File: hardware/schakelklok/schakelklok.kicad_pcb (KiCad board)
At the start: 2 copper layers, 35 parts, among them J1 UART_interface, J2 schakeluitgangen, J3 programmer_1, J4 programmer_2, Q1 BD439, Q2 BD439, Q3 BD439, Q4 BD439, Q5 BD439, SW1 Rotary_Encoder_Switch, U1 24LC64, U2 stm32_bluepill, U3 nrf24l01

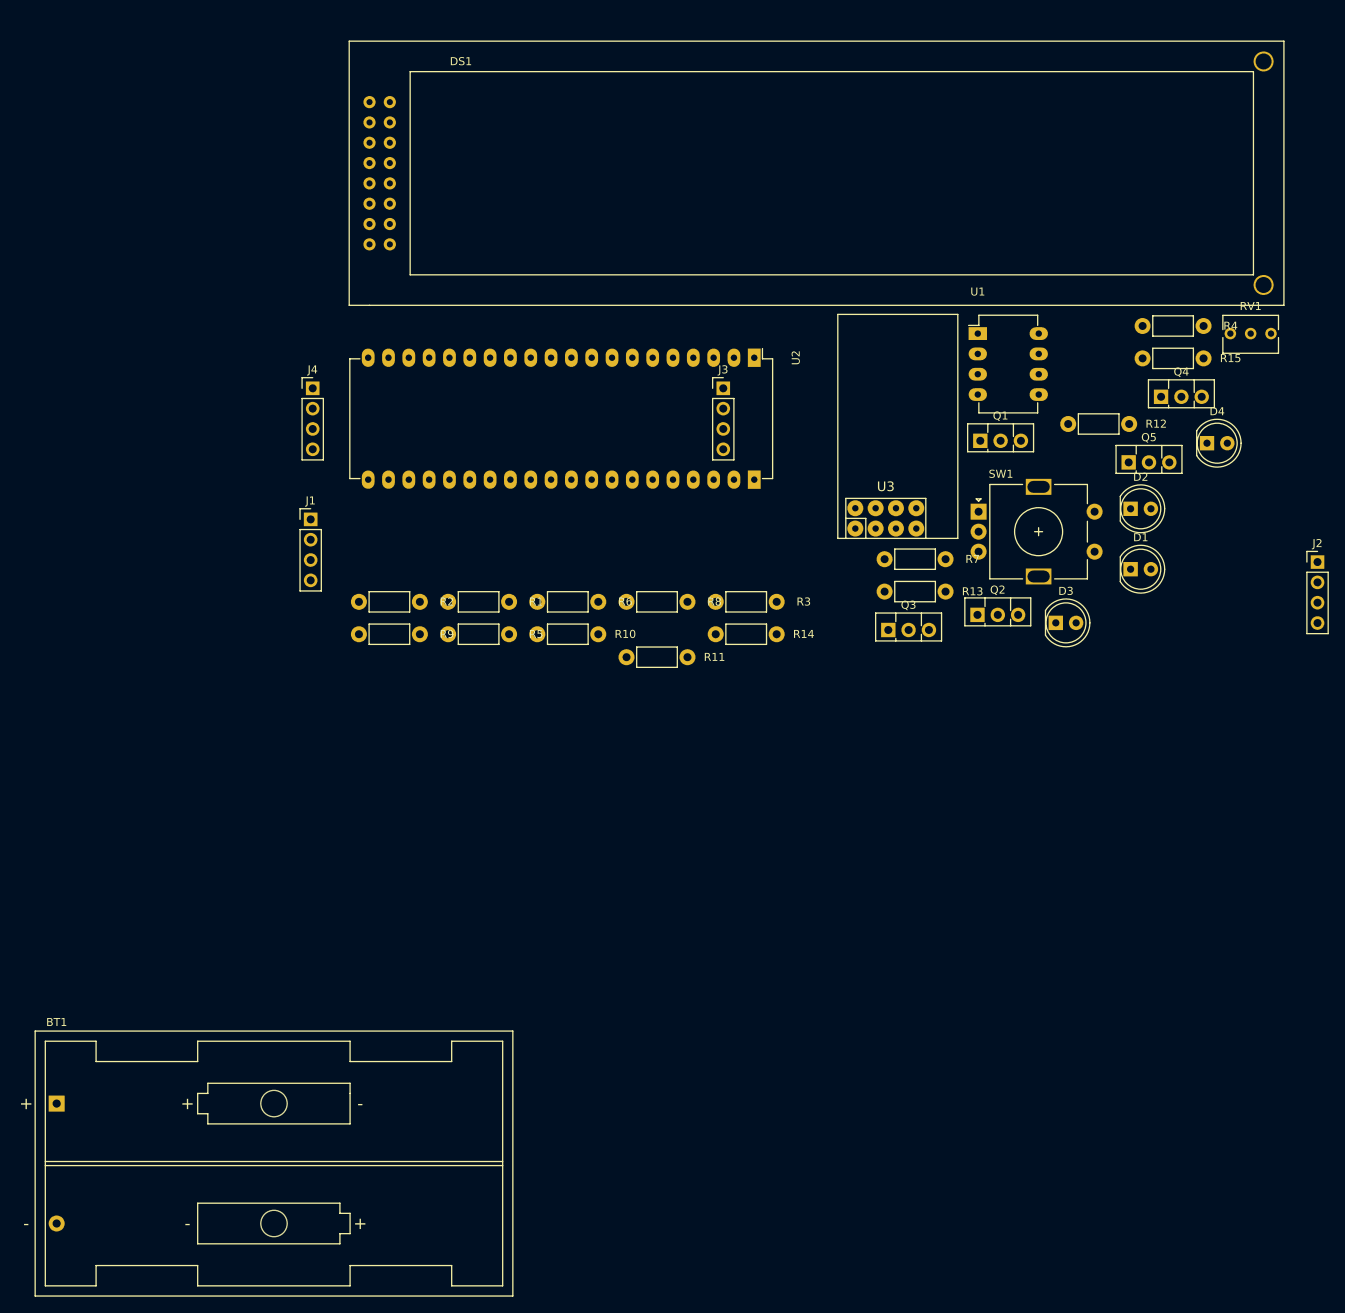
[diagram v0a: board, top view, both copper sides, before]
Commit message: finished hardware
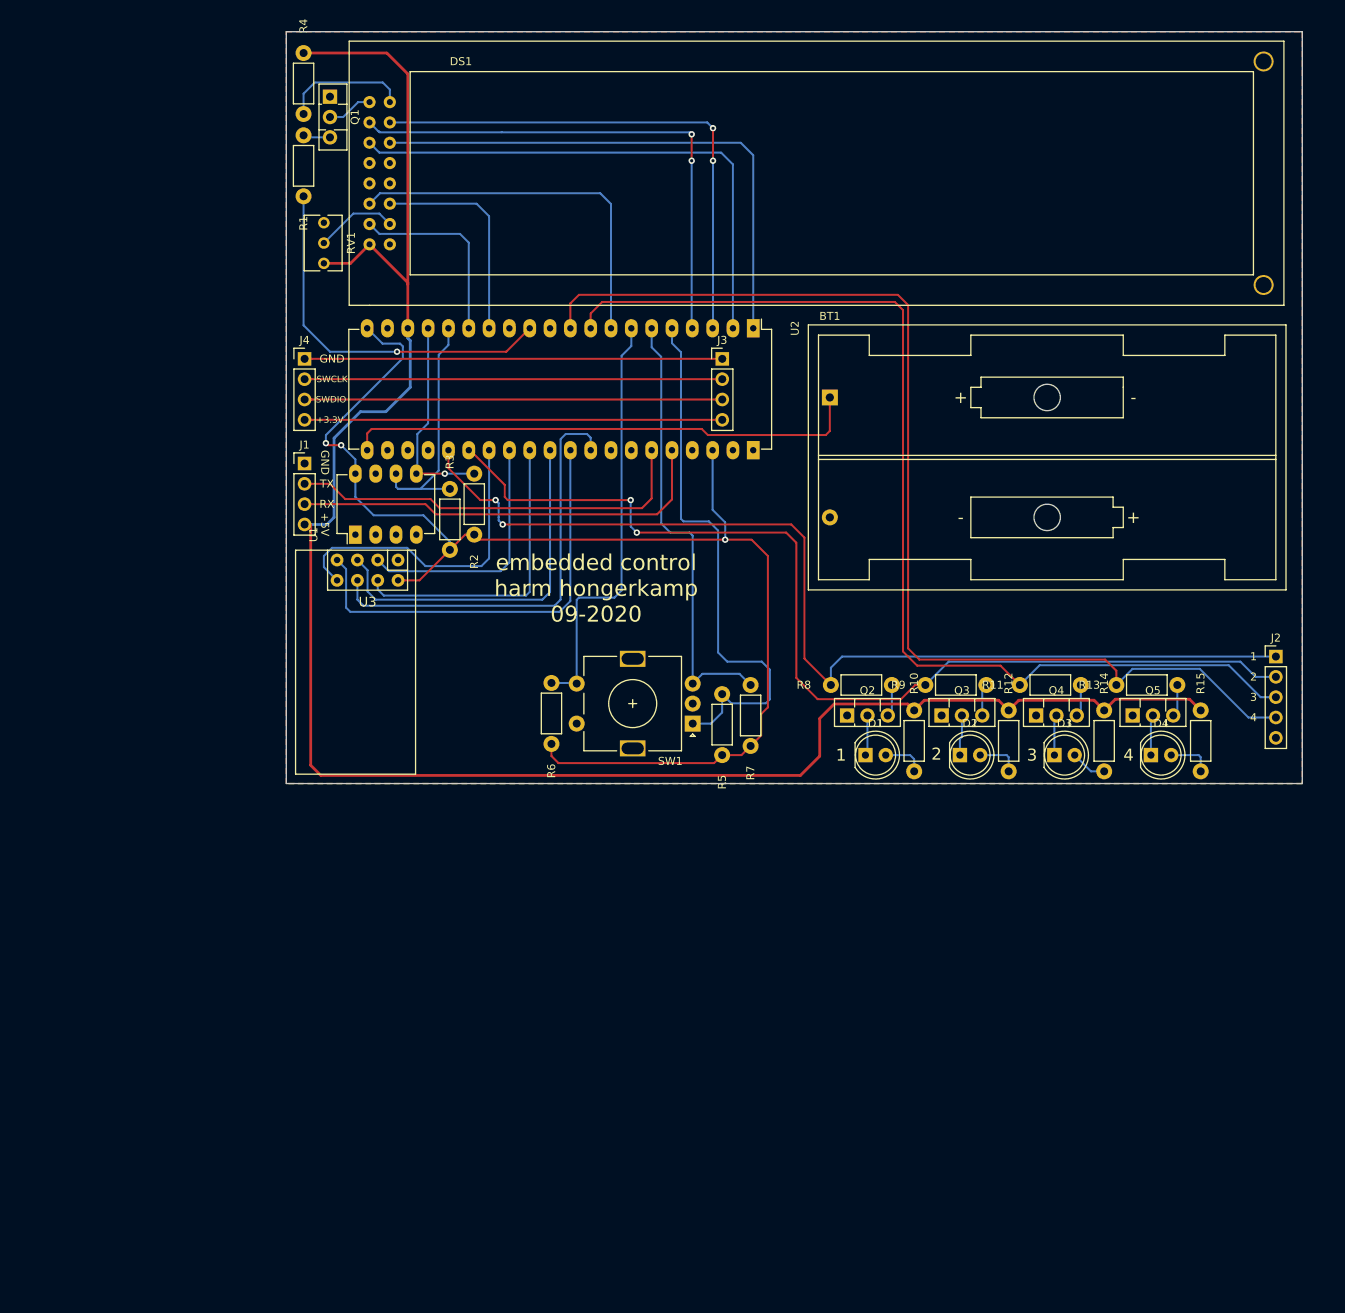
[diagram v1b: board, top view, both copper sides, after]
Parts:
- J2: value schakeluitgangen -> Conn_01x05; footprint Connector_PinHeader_2.54mm:PinHeader_1x04_P2.54mm_Vertical -> Connector_PinHeader_2.54mm:PinHeader_1x05_P2.54mm_Vertical
- moved BT1 130.9 mm to (118.7, 83.8)
- moved RV1 118.7 mm to (55.5, 67.1), turned to 270 degrees
- moved R4 108.2 mm to (53.0, 48.4), turned to 90 degrees
- moved Q1 92.0 mm to (56.3, 46.2), turned to 270 degrees
- moved U1 81.8 mm to (59.4, 101.0), turned to 90 degrees
- moved R9 78.7 mm to (138.3, 119.8), turned to 180 degrees
- moved U3 65.1 mm to (61.0, 105.4), turned to 180 degrees
- moved R1 61.0 mm to (53.0, 51.1), turned to 270 degrees
- moved R11 56.9 mm to (150.1, 119.8), turned to 180 degrees
- moved R15 52.1 mm to (165.1, 130.6), turned to 90 degrees
- moved R14 51.5 mm to (153.0, 130.6), turned to 90 degrees
- moved R10 50.1 mm to (129.3, 130.6), turned to 90 degrees
- moved SW1 44.5 mm to (101.6, 124.6), turned to 180 degrees
- moved R12 44.1 mm to (141.1, 130.6), turned to 90 degrees
- moved Q4 42.8 mm to (144.5, 123.6)
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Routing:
- net +5V: track 0.00 -> 244.3 mm
- net +3V3: track 0.00 -> 159.7 mm, vias 0 -> 3
- net schakeluitgang_4: track 0.00 -> 141.6 mm
- net schakeluitgang_3: track 0.00 -> 135.7 mm
- net schakeluitgang_1: track 0.00 -> 129.9 mm, vias 0 -> 2
- net schakeluitgang_2: track 0.00 -> 129.4 mm, vias 0 -> 2
- net pulse_A: track 0.00 -> 69.0 mm
- net D4: track 0.00 -> 67.7 mm
- net D5: track 0.00 -> 67.0 mm
- net D6: track 0.00 -> 65.7 mm, vias 0 -> 2
- net D7: track 0.00 -> 65.2 mm, vias 0 -> 2
- net Net-(BT1-Pad1): track 0.00 -> 64.9 mm
- net pulse_b: track 0.00 -> 56.3 mm
- net /mosi1: track 0.00 -> 54.3 mm
- net /miso1: track 0.00 -> 54.1 mm
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- added copper zone on B.Cu, net GND
- added copper zone on F.Cu, net GND
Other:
- board outline added: 127 x 94 mm
- net class 5V added: clearance 0.3, trace_width 0.35, via_dia 0.8, via_drill 0.4
- board text added: "+3.3V"
- board text added: "+5V"
- board text added: "1"
- board text added: "2"
- board text added: "3"
- board text added: "4"
- board text added: "GND"
- board text added: "Harm Hongerkamp"
- board text added: "RX"
- board text added: "SWCLK"
- board text added: "SWDIO"
- board text added: "TX"
- board text added: "embedded control harm hongerkamp 09-2020"
